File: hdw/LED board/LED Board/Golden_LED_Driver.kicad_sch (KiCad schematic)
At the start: 20 parts, among them U2 TLC59401RHBR

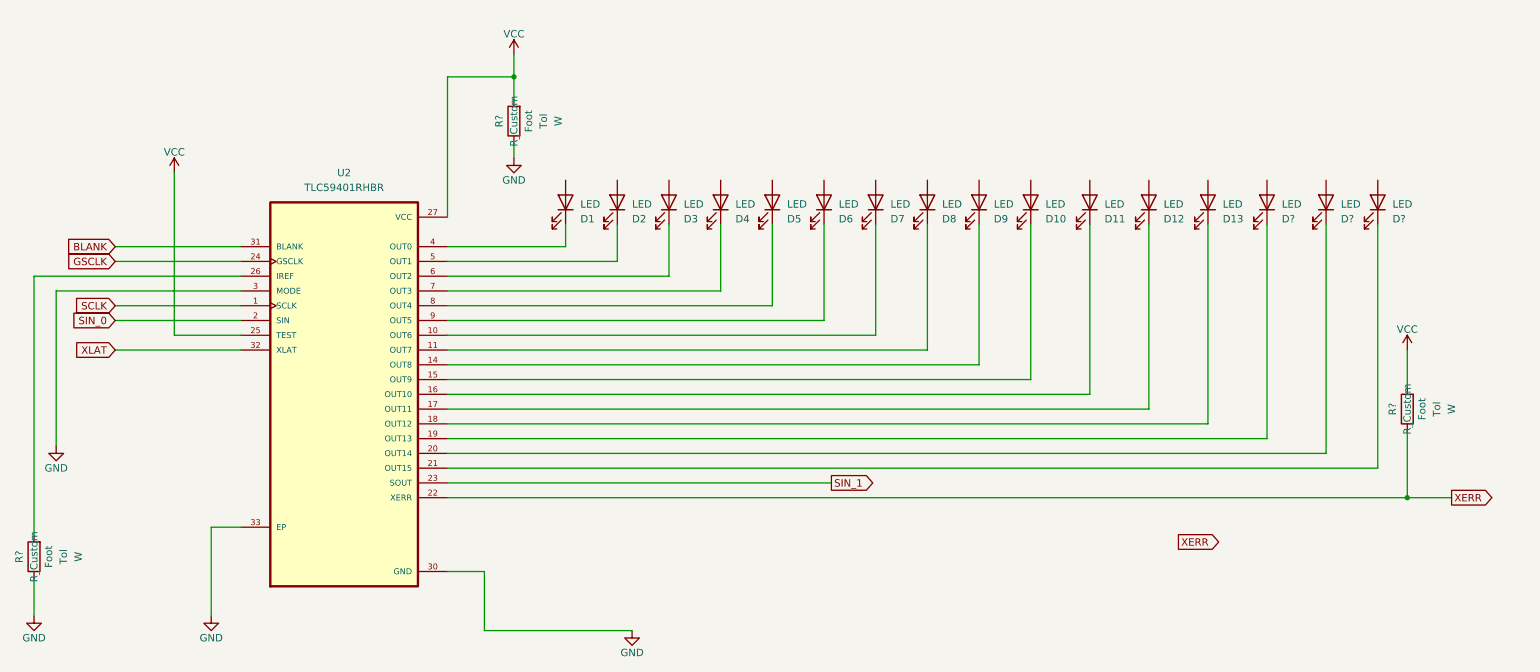
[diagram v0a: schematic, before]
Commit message: new LED driver
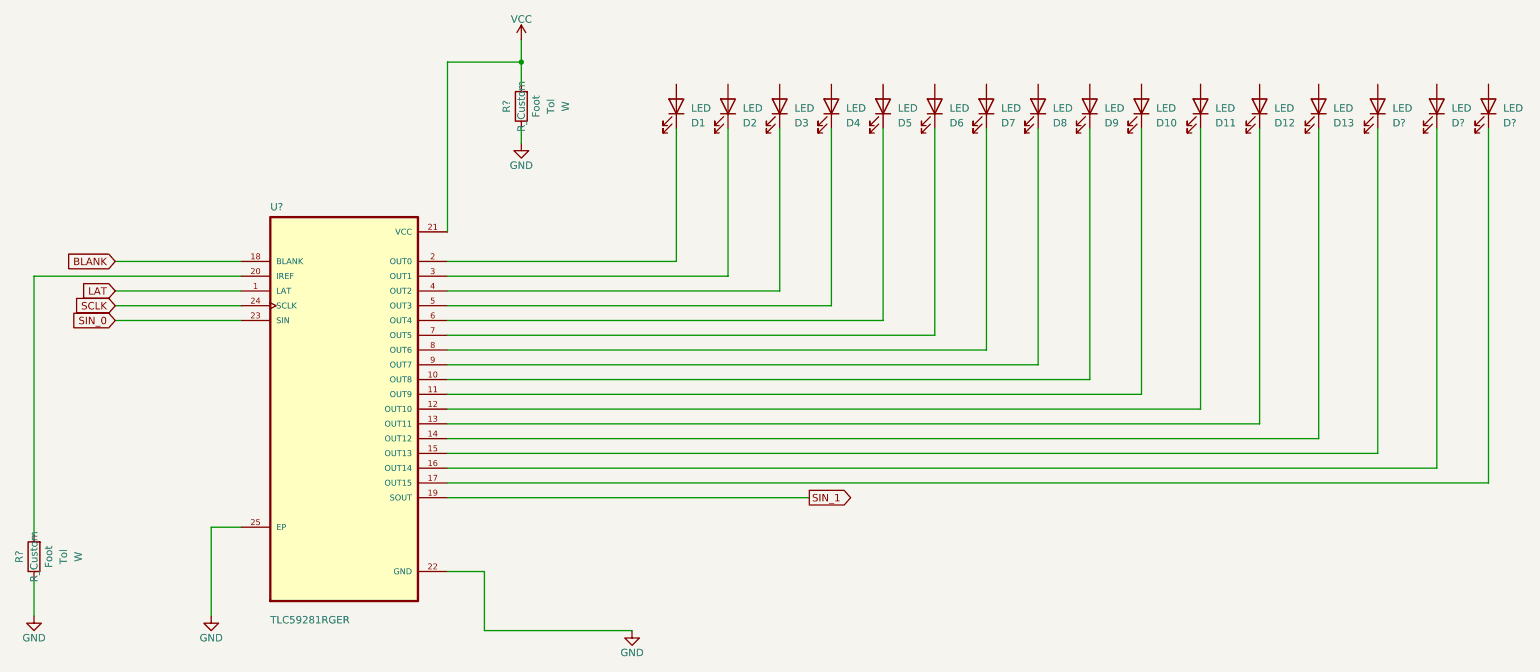
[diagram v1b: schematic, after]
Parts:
- removed R?: R_Custom, Resistor_THT:R_Array_SIP4, symbol Custom Library:R_Custom
- removed U2: TLC59401RHBR, TLC59401RHBR:IC_ADS125H01IRHBT, symbol TLC59401RHBR:TLC59401RHBR
- added U?: TLC59281RGER, TLC59281RGER:QFN50P400X400X100-25N, symbol TLC59281RGER:TLC59281RGER
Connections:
- net BLANK: now also U?.18 (BLANK)
- net GND: now also U?.22 (GND), U?.25 (EP)
- net SCLK: now also U?.24 (SCLK)
- net SIN_0: now also U?.23 (SIN)
- net SIN_1: now also U?.19 (SOUT)
- net VCC: now also U?.21 (VCC)
- net at R?.1: now also U?.20 (IREF)
- net at D6.1 (K): now also U?.7 (OUT5)
- net at D3.1 (K): now also U?.4 (OUT2)
- net at D11.1 (K): now also U?.12 (OUT10)
- net at D7.1 (K): now also U?.8 (OUT6)
- net at D8.1 (K): now also U?.9 (OUT7)
- net at D9.1 (K): now also U?.10 (OUT8)
- net at D10.1 (K): now also U?.11 (OUT9)
- net at D12.1 (K): now also U?.13 (OUT11)
- net at D13.1 (K): now also U?.14 (OUT12)
- net at D?.1 (K): now also U?.15 (OUT13)
- net at D?.1 (K): now also U?.16 (OUT14)
- net at D?.1 (K): now also U?.17 (OUT15)
- net at D1.1 (K): now also U?.2 (OUT0)
- net at D2.1 (K): now also U?.3 (OUT1)
- net at D4.1 (K): now also U?.5 (OUT3)
- net at D5.1 (K): now also U?.6 (OUT4)
- new net LAT: U?.1 (LAT)
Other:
- moved on the sheet: D1, D10, D11, D12, D13, D2, D3, D4, D5, D6, D7, D8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
